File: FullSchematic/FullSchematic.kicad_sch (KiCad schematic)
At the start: 2 parts, among them J3 Conn_01x03_Pin, Q1 PMOS

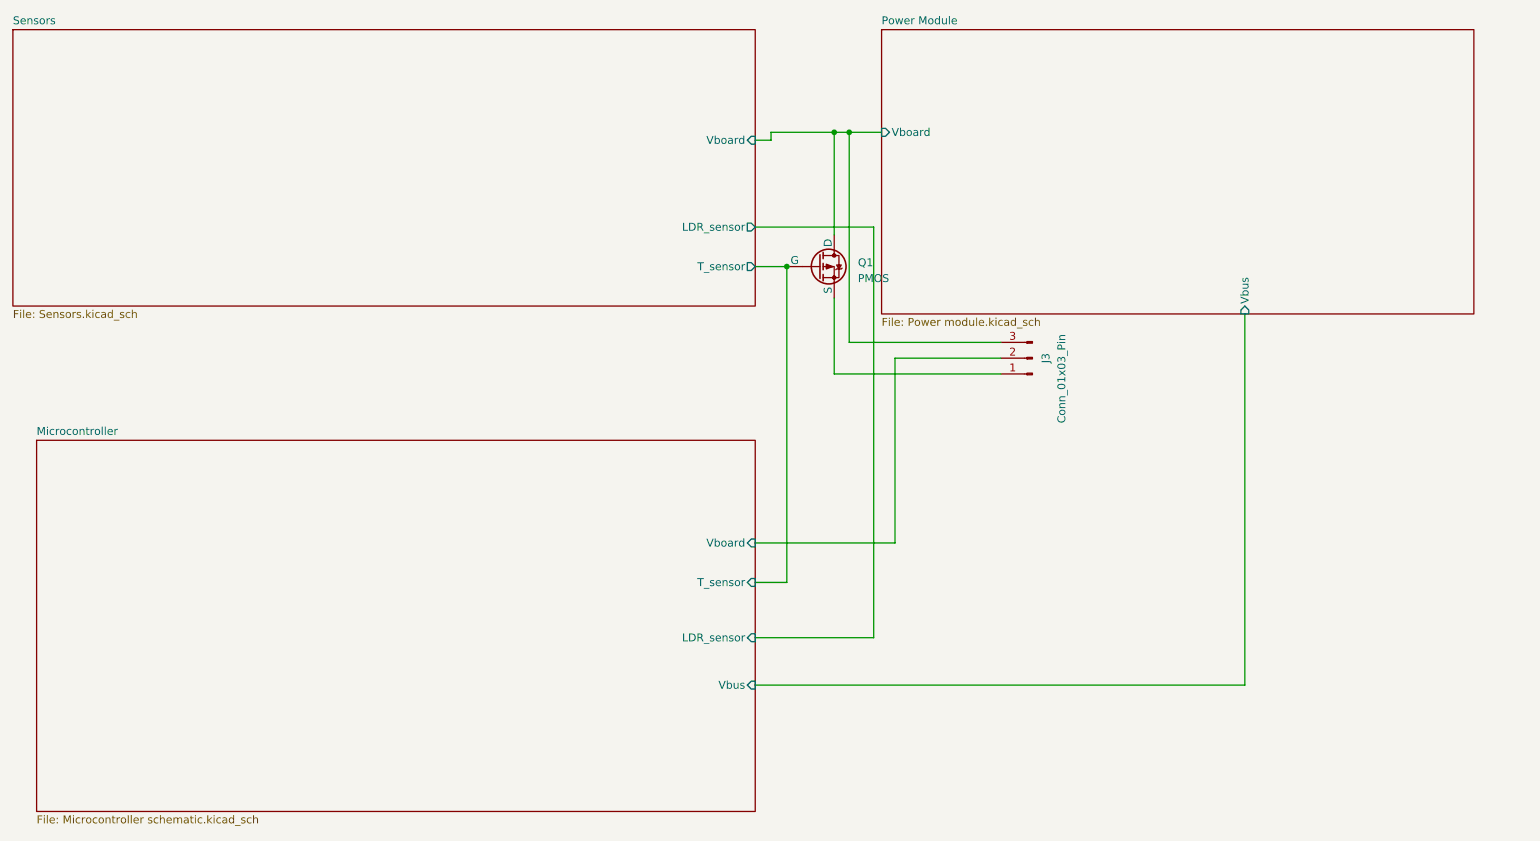
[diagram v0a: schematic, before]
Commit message: Confirmed part numbers and prices
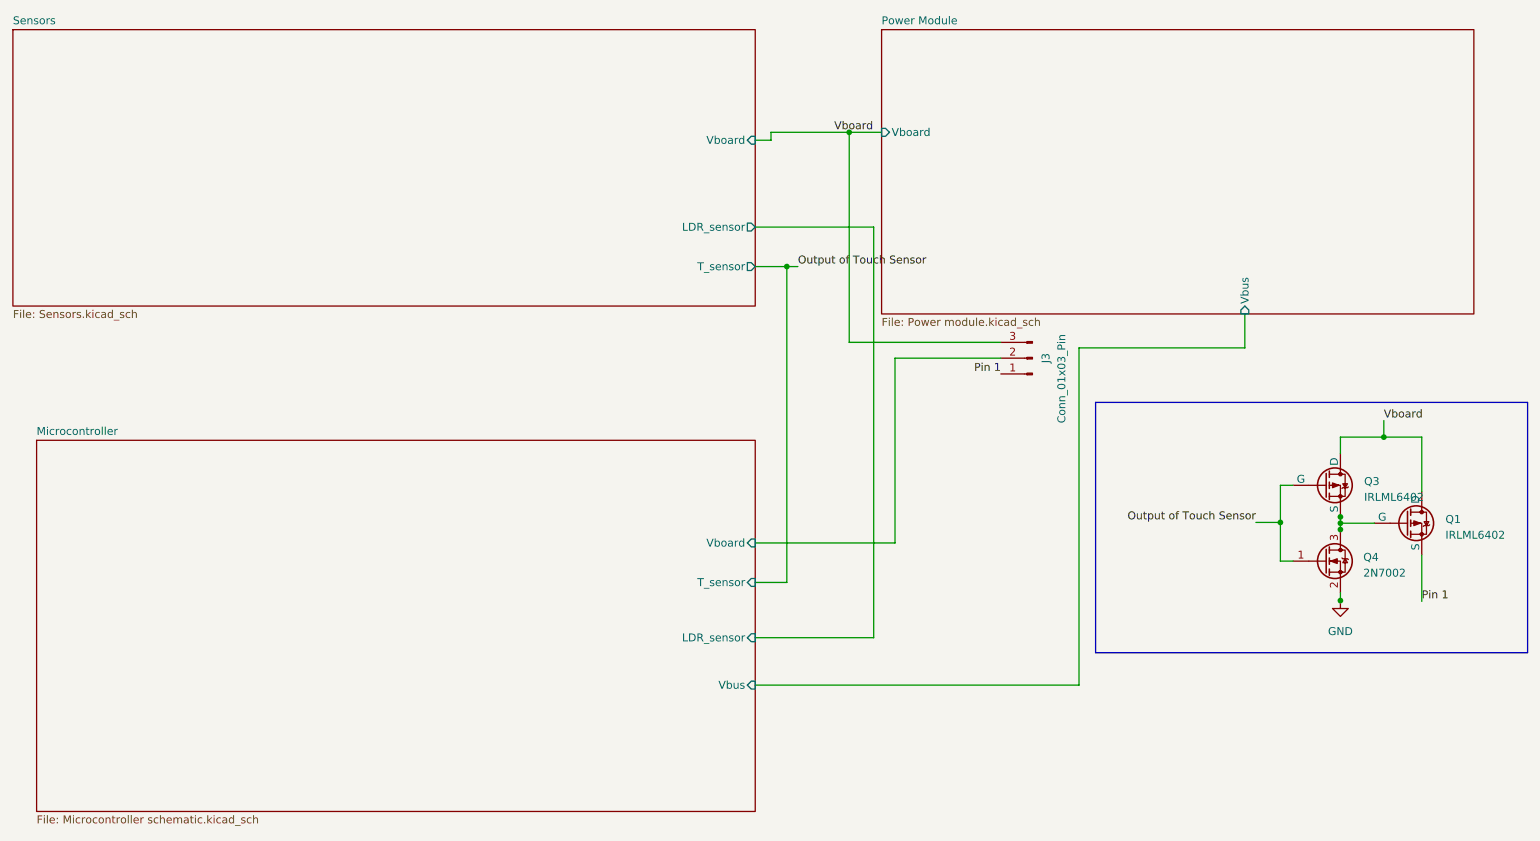
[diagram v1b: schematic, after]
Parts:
- added Q3: IRLML6402, Package_TO_SOT_SMD:SOT-23, symbol Simulation_SPICE:PMOS
- added Q4: 2N7002, Package_TO_SOT_SMD:SOT-23, symbol Transistor_FET:2N7002
- J3: footprint Connector_PinHeader_1.00mm:PinHeader_1x03_P1.00mm_Vertical -> Connector_PinHeader_2.54mm:PinHeader_1x03_P2.54mm_Vertical; JLCPCB Part # (none) -> N/A; Populate (none) -> No; Price (none) -> N/A; Price ( 1 board) (none) -> N/A; Price (5 boards) (none) -> N/A
- Q1: value PMOS -> IRLML6402; footprint Package_TO_SOT_THT:TO-3P-3_Vertical -> Package_TO_SOT_SMD:SOT-23; JLCPCB Part # C115991 -> C518785; Populate (none) -> Yes; Price 0.52 -> 0.5; Price ( 1 board) 0.52 -> 0.5; Price (5 boards) 2.6 -> 0.25
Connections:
- net Pin 1: now reaches J3.1 (Pin_1), Q1.3 (S)
- net Microcontroller/T_sensor: no longer names the net of Q1.2 (G)
- net Microcontroller/T_sensor: now also Q3.3 (S), Q4.3 (D)
- net Power Module/Vboard renamed Vboard
- net Vboard: now also Q3.1 (D)
- new net GND: Q4.2 (S)
- new net Output of Touch Sensor: Q3.2 (G), Q4.1 (G)
